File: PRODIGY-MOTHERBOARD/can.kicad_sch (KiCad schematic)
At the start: 1 part, among them U9 SN65HVD232

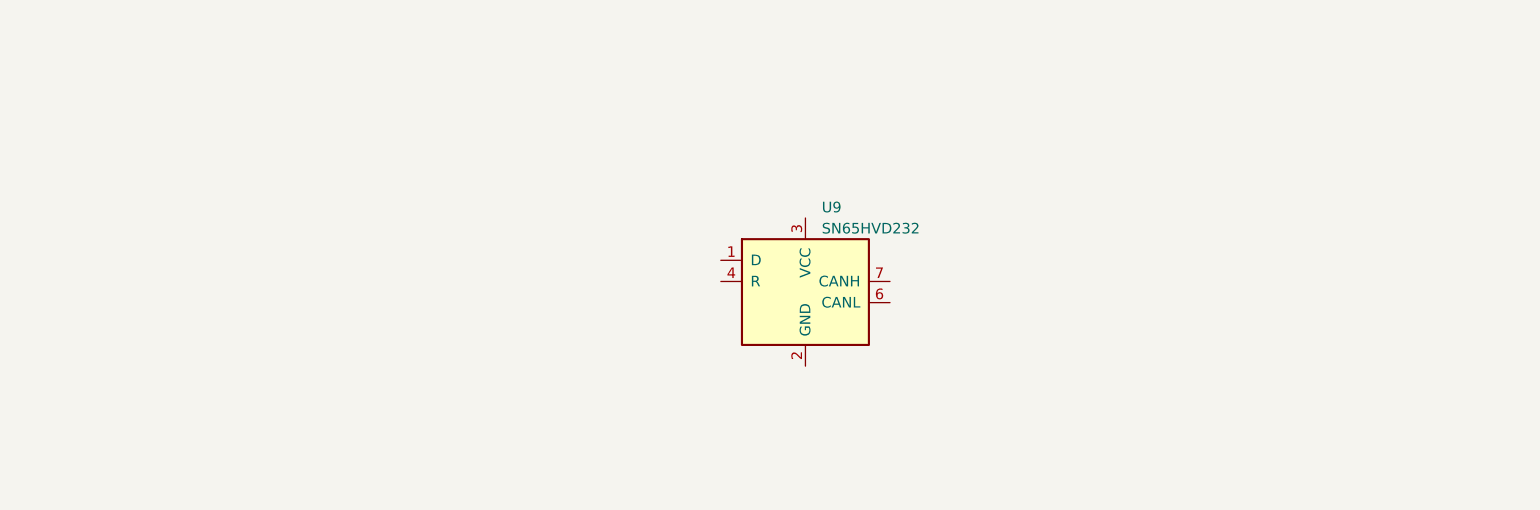
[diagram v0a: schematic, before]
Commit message: CAN schematic done
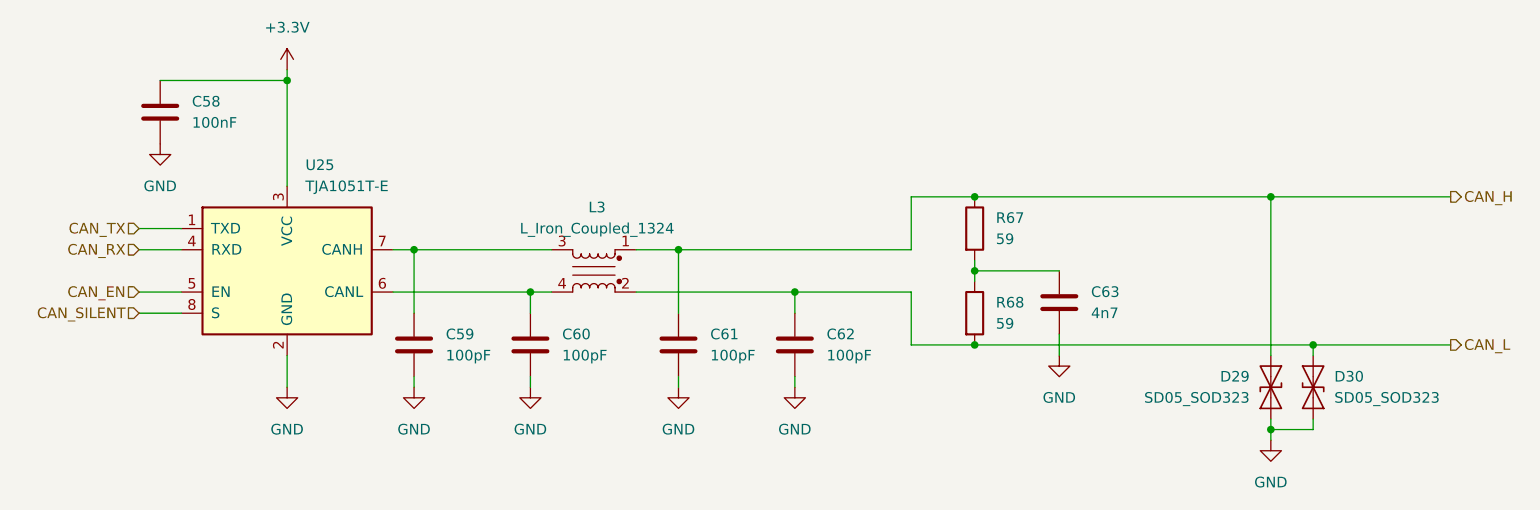
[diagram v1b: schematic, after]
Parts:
- removed U9: SN65HVD232, Package_SO:SOIC-8_3.9x4.9mm_P1.27mm, symbol Interface_CAN_LIN:SN65HVD232
- added C58: 100nF, Capacitor_SMD:C_0603_1608Metric, symbol Device:C
- added C59, C60, C61, C62: 100pF, symbol Device:C
- added C63: 4n7, symbol Device:C
- added D29, D30: SD05_SOD323, Diode_SMD:D_SOD-323, symbol Diode:SD05_SOD323
- added L3: L_Iron_Coupled_1324, Inductor_SMD:L_CommonModeChoke_TDK_ACM7060, symbol Device:L_Iron_Coupled_1324
- added R67, R68: 59, Resistor_SMD:R_1206_3216Metric, symbol Device:R
- added U25: TJA1051T-E, Package_SO:SOIC-8_3.9x4.9mm_P1.27mm, symbol Interface_CAN_LIN:TJA1051T-E
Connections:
- new net: C60.1, L3.4, U25.6 (CANL)
- new net: C63.1, R67.2, R68.1
- new net: C59.1, L3.3, U25.7 (CANH)
- new net +3.3V: C58.1, U25.3 (VCC)
- new net CAN_EN: U25.5 (EN)
- new net CAN_H: C61.1, D29.2 (A2), L3.1, R67.1
- new net CAN_L: C62.1, D30.2 (A2), L3.2, R68.2
- new net CAN_RX: U25.4 (RXD)
- new net CAN_SILENT: U25.8 (S)
- new net CAN_TX: U25.1 (TXD)
- new net GND: C58.2, C59.2, C60.2, C61.2, C62.2, C63.2, D29.1 (A1), D30.1 (A1), U25.2 (GND)
